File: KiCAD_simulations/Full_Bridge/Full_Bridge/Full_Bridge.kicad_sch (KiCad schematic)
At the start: 7 parts

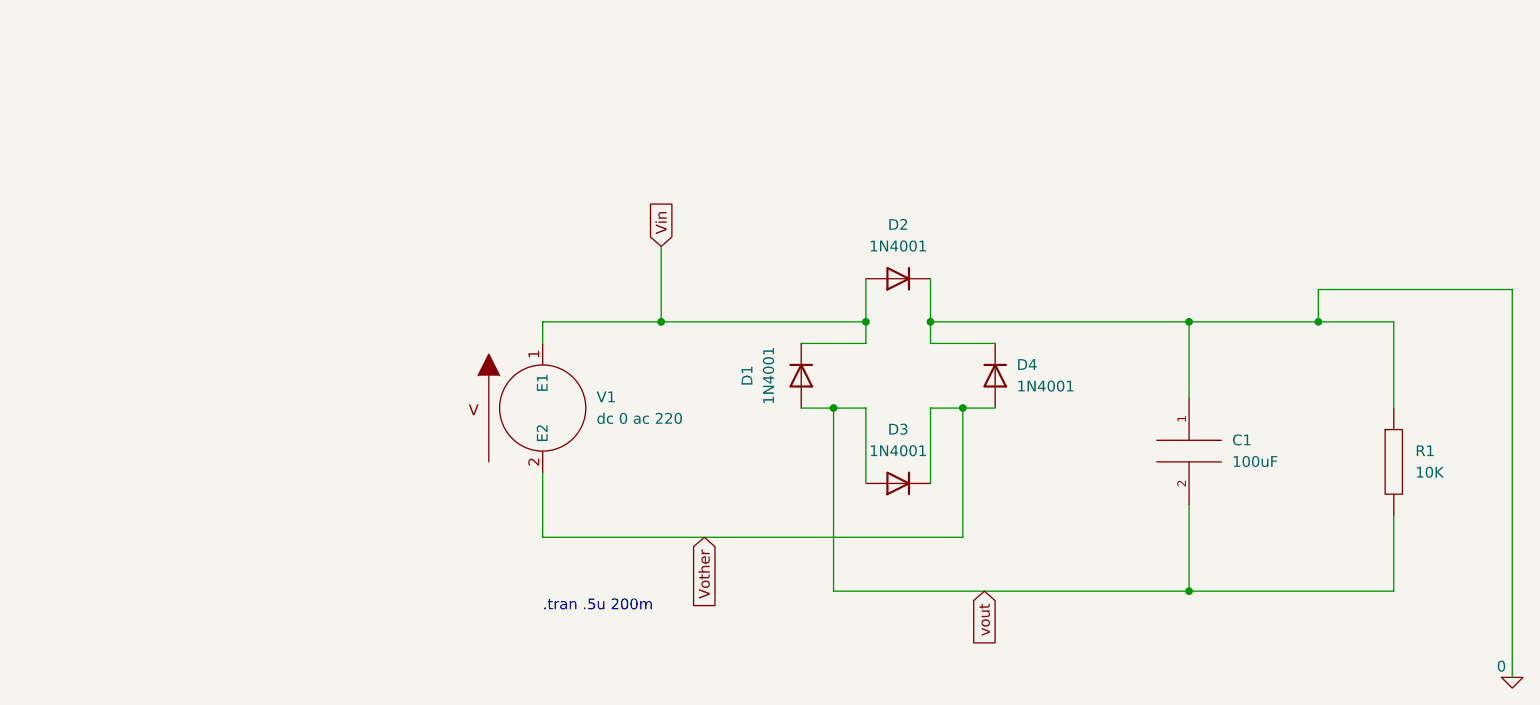
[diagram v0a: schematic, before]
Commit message: updates
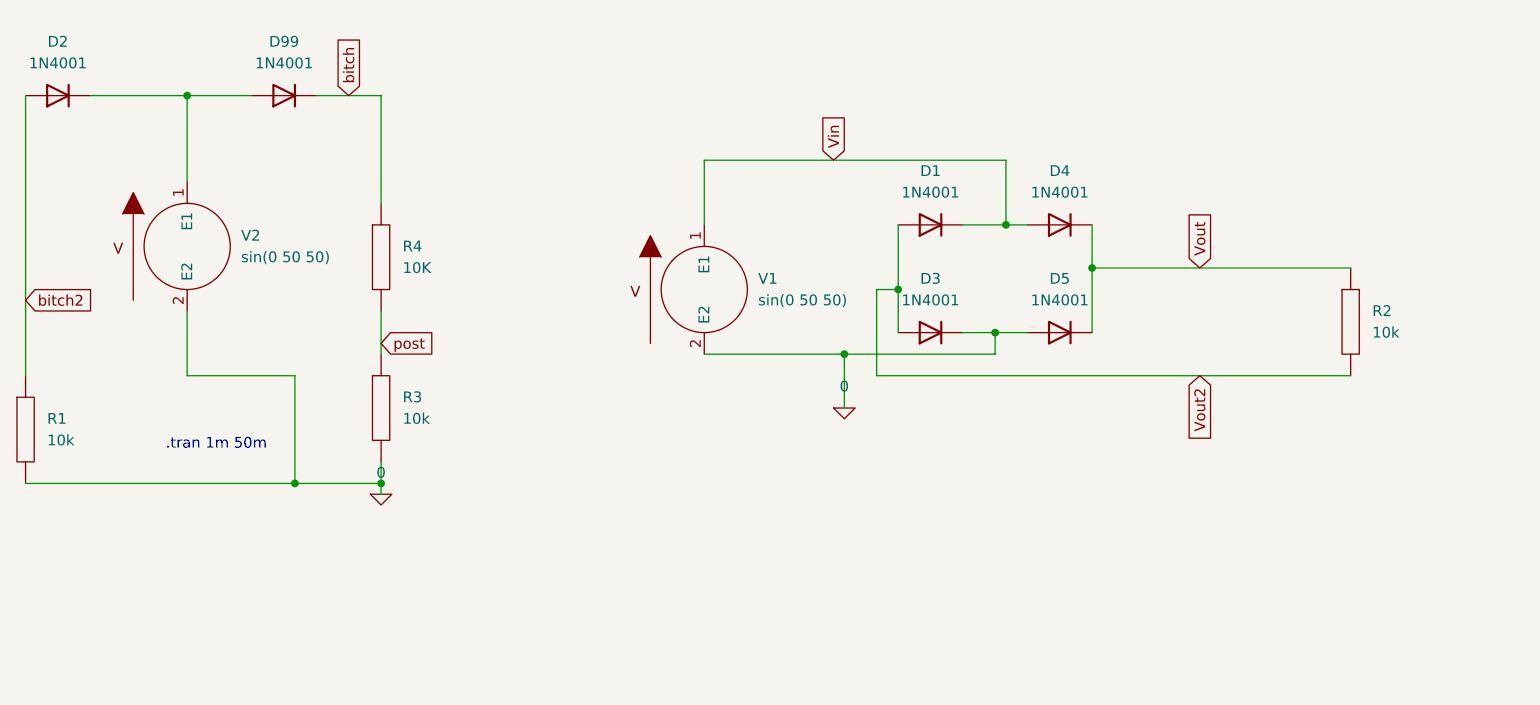
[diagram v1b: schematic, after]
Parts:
- removed C1: 100uF, symbol pspice:C
- added D5, D99: 1N4001, Diode_THT:D_DO-41_SOD81_P10.16mm_Horizontal, symbol Diode:1N4001
- added R2, R3: 10k, symbol pspice:R
- added R4: 10K, symbol pspice:R
- added V2: sin(0 50 50), symbol pspice:VSOURCE
- D1, D2, D3: Spice_Node_Sequence (none) -> 2 1
- R1: value 10K -> 10k
- V1: value dc 0 ac 220 -> sin(0 50 50); Spice_Model dc 0 ac 20 sin(0 220 50 0) -> (none); Spice_Netlist_Enabled Y -> (none); Spice_Primitive V -> (none)
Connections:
- net 0: now also D3.1 (K), R1.2, V1.2 (E2), D5.2 (A), R3.2, V2.2 (E2); no longer D2.1 (K), D4.1 (K), R1.1
- net Vin: now also D4.2 (A); no longer D2.2 (A)
- removed net Vother: D3.1 (K), D4.2 (A), V1.2 (E2)
- net vout renamed Vout2
- net Vout2: now also R2.2; no longer R1.2
- new net: D2.1 (K), D99.2 (A), V2.1 (E1)
- new net Vout: D4.1 (K), D5.1 (K), R2.1
- new net bitch: D99.1 (K), R4.1
- new net bitch2: D2.2 (A), R1.1
- new net post: R3.1, R4.2
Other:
- note added: ".tran 1m 50m"
- note removed: ".tran .5u 200m"
